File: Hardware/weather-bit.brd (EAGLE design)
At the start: 68.6 x 67.3 mm, 40 parts, among them J2 RJ11, J3 RJ11, U1 BME280, U2 micro:bit

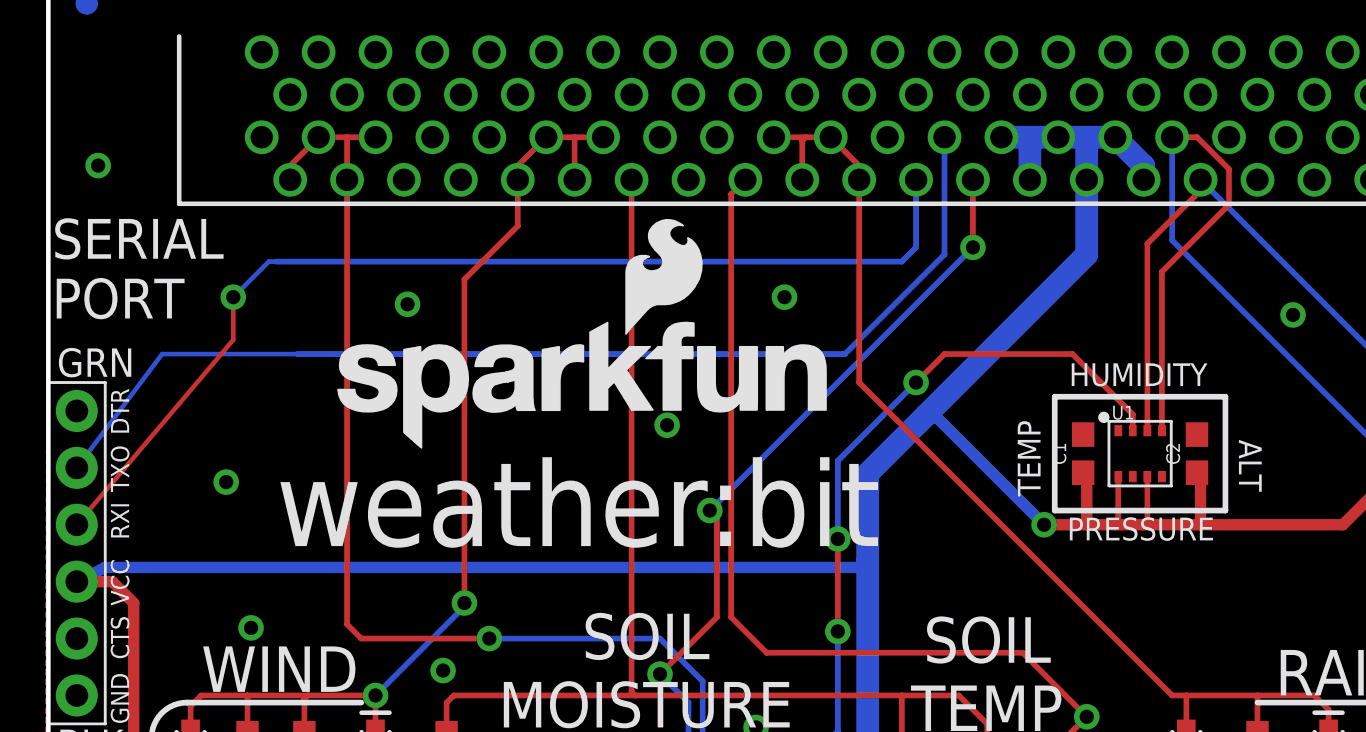
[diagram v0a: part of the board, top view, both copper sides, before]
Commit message: Updated BRD and SCH files per EDU
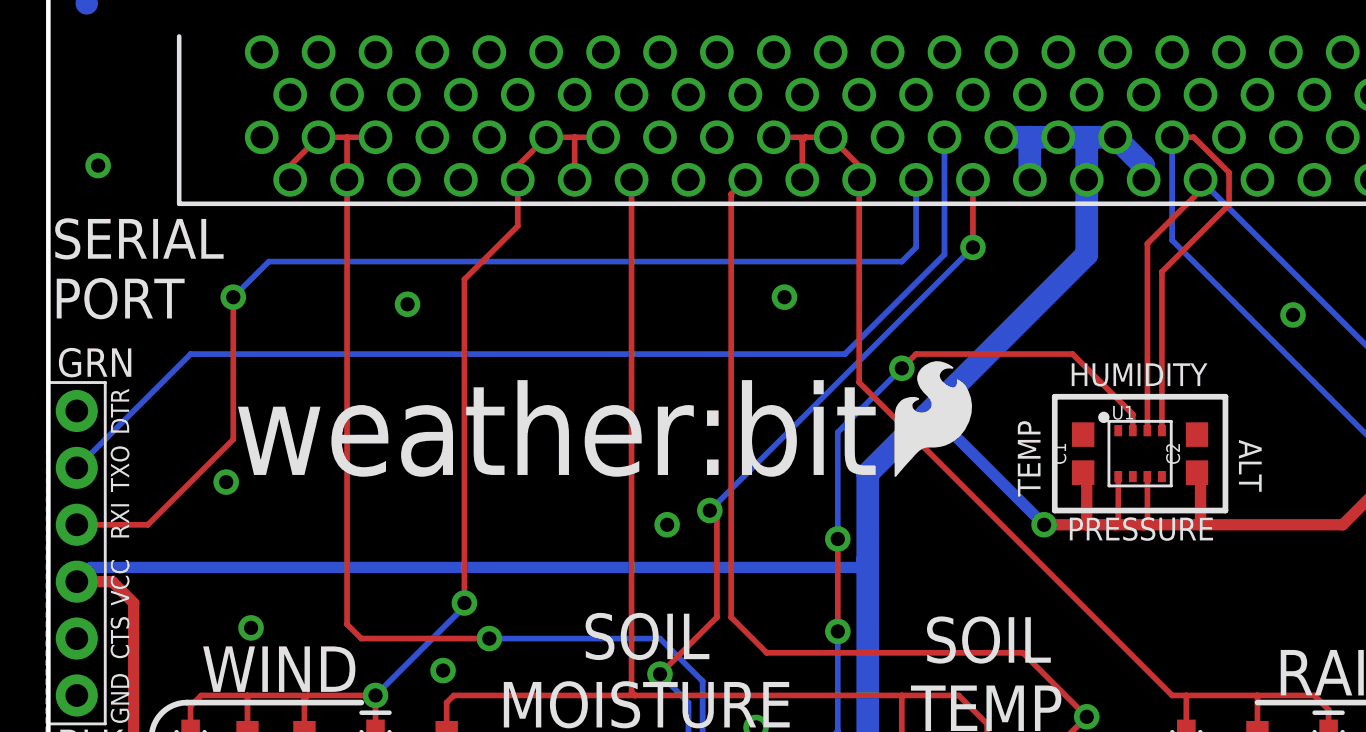
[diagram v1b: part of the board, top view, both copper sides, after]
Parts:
- removed LOGO1: SFE_LOGO_NAME_FLAME.2_INCH, SparkFun-Aesthetics:SFE_LOGO_NAME_FLAME_.2
- added U$1: (no value), SparkFun-Aesthetics:SFE_LOGO_FLAME_.2
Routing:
- net RXI: track 47.1 -> 49.3 mm
- net N$2: track 36.5 -> 37.2 mm
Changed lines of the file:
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@@
 <setting verticaltext="up"/>
 </settings>
-<grid distance="0.025" unitdist="inch" unit="inch" style="dots" multiple="1" display="yes" altdistance="0.0001" altunitdist="inch" altunit="inch"/>
+<grid distance="0.0001" unitdist="inch" unit="inch" style="dots" multiple="1" display="yes" altdistance="0.0001" altunitdist="inch" altunit="inch"/>
 <layers>
 <layer number="1" name="Top" color="4" fill="1" visible="yes" active="yes"/>
@@
 <text x="6.82625" y="23.01875" size="2.032" layer="21" ratio="15">WIND</text>
 <text x="54.76875" y="22.86" size="2.032" layer="21" ratio="15">RAIN</text>
-<text x="10.16" y="29.5275" size="3.81" layer="21" ratio="20">weather:bit</text>
+<text x="8.255" y="32.7025" size="4.064" layer="21" ratio="20">weather:bit</text>
 <text x="24.4475" y="8.09625" size="1.27" layer="21" ratio="15" rot="R180">VCC</text>
 <text x="28.575" y="8.09625" size="1.27" layer="21" ratio="15" rot="R180">GND</text>
@@
 <attribute name="PROD_ID" value="RES-07857" x="45.085" y="19.05" size="1.778" layer="27" rot="R270" display="off"/>
 </element>
-<element name="LOGO1" library="SparkFun-Aesthetics" package="SFE_LOGO_NAME_FLAME_.2" value="SFE_LOGO_NAME_FLAME.2_INCH" x="12.22375" y="33.81375"/>
 <element name="H3" library="SparkFun-Electromechanical" package="STAND-OFF" value="STAND-OFF" x="2.54" y="2.54"/>
 <element name="H4" library="SparkFun-Electromechanical" package="STAND-OFF" value="STAND-OFF" x="66.04" y="2.54"/>
@@
 </element>
 <element name="J1" library="SparkFun-Connectors" package="6_PIN_SERIAL_TARGET_SIDE_W_SILK" value="" x="1.27" y="29.21" rot="R270"/>
+<element name="U$1" library="SparkFun-Aesthetics" package="SFE_LOGO_FLAME_.2" value="" x="37.465" y="32.385"/>
 </elements>
 <signals>
@@
 <contactref element="J9" pad="4"/>
 <via x="32.86125" y="40.64" extent="1-16" drill="0.635"/>
-<via x="27.6225" y="34.925" extent="1-16" drill="0.635"/>
+<via x="27.6225" y="30.48" extent="1-16" drill="0.635"/>
 <via x="65.56375" y="12.54125" extent="1-16" drill="0.635"/>
 <via x="66.04" y="54.2925" extent="1-16" drill="0.635"/>
@@
 <wire x1="41.3385" y1="16.1925" x2="41.91" y2="16.764" width="0.508" layer="1"/>
 <wire x1="36.2585" y1="28.575" x2="36.576" y2="28.8925" width="0.508" layer="16"/>
-<wire x1="36.2585" y1="28.575" x2="2.54" y2="28.575" width="0.508" layer="16"/>
-<wire x1="2.54" y1="28.575" x2="1.27" y2="27.94" width="0.508" layer="16"/>
+<wire x1="36.2585" y1="28.575" x2="1.905" y2="28.575" width="0.508" layer="16"/>
 <wire x1="1.27" y1="27.94" x2="2.8575" y2="27.94" width="0.508" layer="1"/>
 <wire x1="2.8575" y1="27.94" x2="3.81" y2="26.9875" width="0.508" layer="1"/>
@@
 <wire x1="41.91" y1="17.9" x2="41.91" y2="16.9545" width="0.508" layer="1"/>
 <wire x1="41.91" y1="16.9545" x2="42.00525" y2="16.85925" width="0.508" layer="1"/>
+<wire x1="1.905" y1="28.575" x2="1.27" y2="27.94" width="0.508" layer="16"/>
 </signal>
 <signal name="N$2">
@@
 <wire x1="29.21" y1="18.0975" x2="30.1625" y2="18.0975" width="0.254" layer="1"/>
 <wire x1="29.21" y1="18.0975" x2="29.21" y2="18.2" width="0.254" layer="1"/>
-<via x="38.735" y="36.83" extent="1-16" drill="0.635"/>
+<via x="38.1" y="37.465" extent="1-16" drill="0.635"/>
 <via x="35.2425" y="29.845" extent="1-16" drill="0.635"/>
 <via x="35.2425" y="25.7175" extent="1-16" drill="0.635"/>
@@
 <wire x1="48.41125" y1="34.68" x2="48.41125" y2="35.40875" width="0.254" layer="1"/>
 <wire x1="48.41125" y1="35.40875" x2="45.72" y2="38.1" width="0.254" layer="1"/>
-<wire x1="45.72" y1="38.1" x2="40.005" y2="38.1" width="0.254" layer="1"/>
-<wire x1="40.005" y1="38.1" x2="38.735" y2="36.83" width="0.254" layer="1"/>
-<wire x1="35.2425" y1="29.845" x2="35.2425" y2="33.3375" width="0.254" layer="16"/>
-<wire x1="35.2425" y1="33.3375" x2="38.735" y2="36.83" width="0.254" layer="16"/>
+<wire x1="45.72" y1="38.1" x2="38.735" y2="38.1" width="0.254" layer="1"/>
+<wire x1="35.2425" y1="29.845" x2="35.2425" y2="34.6075" width="0.254" layer="16"/>
 <wire x1="35.2425" y1="25.7175" x2="35.2425" y2="21.2725" width="0.254" layer="16"/>
 <wire x1="35.2425" y1="21.2725" x2="32.7025" y2="18.7325" width="0.254" layer="16"/>
 <wire x1="32.7025" y1="18.7325" x2="30.7975" y2="18.7325" width="0.254" layer="16"/>
+<wire x1="35.2425" y1="34.6075" x2="38.1" y2="37.465" width="0.254" layer="16"/>
+<wire x1="38.735" y1="38.1" x2="38.1" y2="37.465" width="0.254" layer="1"/>
 </signal>
 <signal name="SDA">
@@
 <contactref element="J9" pad="1"/>
 <contactref element="U2" pad="A8"/>
-<wire x1="50.165" y1="47.77875" x2="51.28125" y2="47.77875" width="0.254" layer="1"/>
-<wire x1="51.28125" y1="47.77875" x2="52.705" y2="46.355" width="0.254" layer="1"/>
-<wire x1="52.705" y1="46.355" x2="52.705" y2="44.7675" width="0.254" layer="1"/>
 <wire x1="52.705" y1="44.7675" x2="49.71125" y2="41.77375" width="0.254" layer="1"/>
 <wire x1="49.71125" y1="34.68" x2="49.71125" y2="41.77375" width="0.254" layer="1"/>
@@
 <wire x1="50.165" y1="43.18" x2="64.135" y2="29.21" width="0.254" layer="16"/>
 <wire x1="64.135" y1="29.21" x2="67.31" y2="29.21" width="0.254" layer="16"/>
+<wire x1="50.165" y1="47.77875" x2="51.12885" y2="47.77875" width="0.254" layer="1"/>
+<wire x1="51.12885" y1="47.77875" x2="52.705" y2="46.2026" width="0.254" layer="1"/>
+<wire x1="52.705" y1="44.7675" x2="52.705" y2="46.2026" width="0.254" layer="1"/>
 </signal>
 <signal name="N$5">
@@
 <signal name="RXI">
 <wire x1="38.735" y1="42.8625" x2="38.1" y2="42.2275" width="0.254" layer="16"/>
-<wire x1="38.1" y1="42.2275" x2="10.16" y2="42.2275" width="0.254" layer="16"/>
+<wire x1="38.1" y1="42.2275" x2="9.8425" y2="42.2275" width="0.254" layer="16"/>
 <contactref element="U2" pad="A17"/>
 <wire x1="38.735" y1="42.8625" x2="38.735" y2="45.87875" width="0.254" layer="16"/>
 <contactref element="J1" pad="P$3"/>
-<wire x1="10.16" y1="42.2275" x2="9.8425" y2="42.2275" width="0.2032" layer="16"/>
-<wire x1="9.8425" y1="42.2275" x2="8.255" y2="40.64" width="0.2032" layer="16"/>
 <via x="8.255" y="40.64" extent="1-16" drill="0.635"/>
-<wire x1="8.255" y1="40.64" x2="8.255" y2="38.735" width="0.2032" layer="1"/>
-<wire x1="8.255" y1="38.735" x2="1.27" y2="30.48" width="0.2032" layer="1"/>
+<wire x1="8.255" y1="34.29" x2="4.445" y2="30.48" width="0.254" layer="1"/>
+<wire x1="4.445" y1="30.48" x2="1.27" y2="30.48" width="0.254" layer="1"/>
+<wire x1="9.8425" y1="42.2275" x2="8.255" y2="40.64" width="0.254" layer="16"/>
+<wire x1="8.255" y1="34.29" x2="8.255" y2="40.64" width="0.254" layer="1"/>
 </signal>
 <signal name="TXO">
 <wire x1="40.005" y1="42.545" x2="35.56" y2="38.1" width="0.254" layer="16"/>
-<wire x1="35.56" y1="38.1" x2="11.1125" y2="38.1" width="0.254" layer="16"/>
+<wire x1="35.56" y1="38.1" x2="6.35" y2="38.1" width="0.254" layer="16"/>
 <contactref element="U2" pad="A16"/>
 <wire x1="40.005" y1="42.545" x2="40.005" y2="47.77875" width="0.254" layer="16"/>
 <contactref element="J1" pad="P$2"/>
-<wire x1="11.1125" y1="38.1" x2="5.08" y2="38.1" width="0.2032" layer="16"/>
-<wire x1="5.08" y1="38.1" x2="1.27" y2="33.02" width="0.2032" layer="16"/>
+<wire x1="6.35" y1="38.1" x2="1.27" y2="33.02" width="0.254" layer="16"/>
 </signal>
 <signal name="13">
@@
 </signal>
 </signals>
-<errors>
-</errors>
 </board>
 </drawing>
